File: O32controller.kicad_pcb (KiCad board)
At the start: 4 copper layers, 27 x 27 mm, 64 parts, among them J1 Conn_01x08_MountingPin, J2 BATT+, J3 BATT-, J4 Motor Connection, J5 Motor Connection, J6 Motor Connection, J7 BATT+, J8 BATT-, Q1 CSD88584Q5DCT, Q2 CSD88584Q5DCT, Q3 CSD88584Q5DCT, U1 AS5047D, U2 STSPIN32F0A

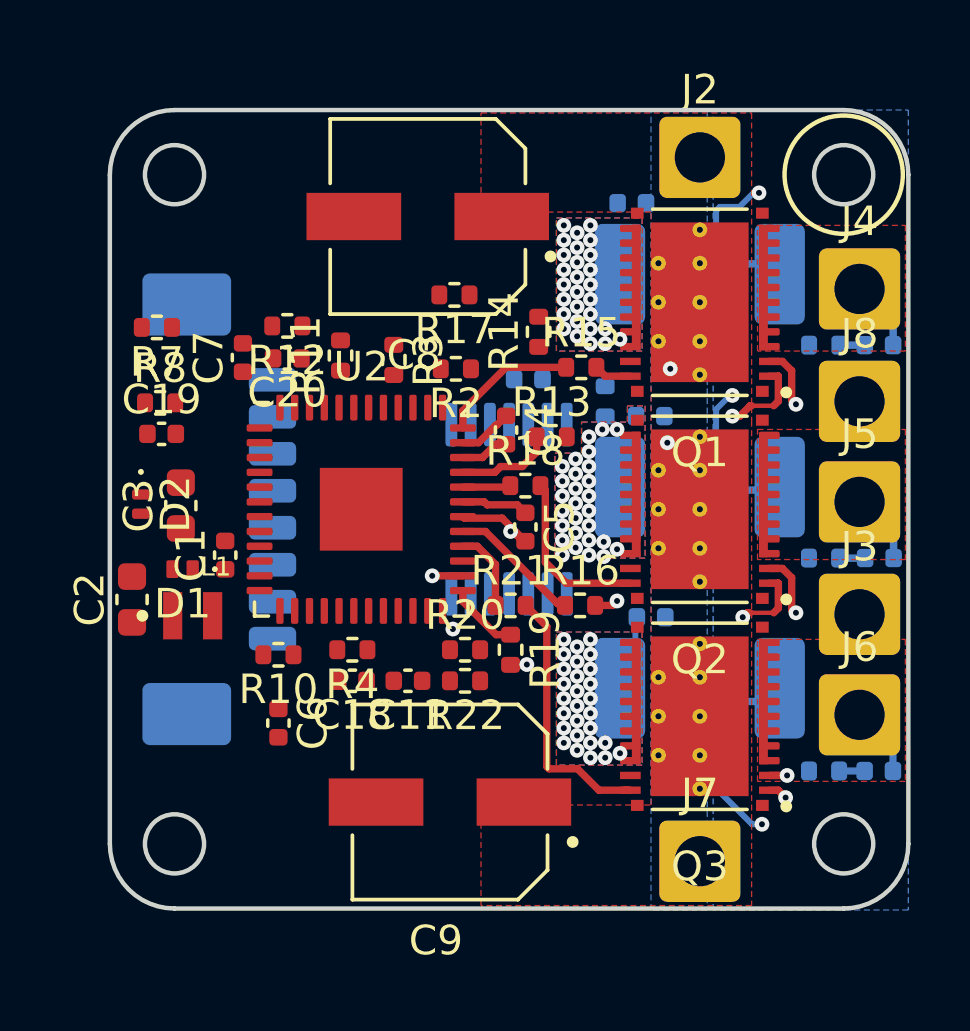
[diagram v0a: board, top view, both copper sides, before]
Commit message: fixed clearances
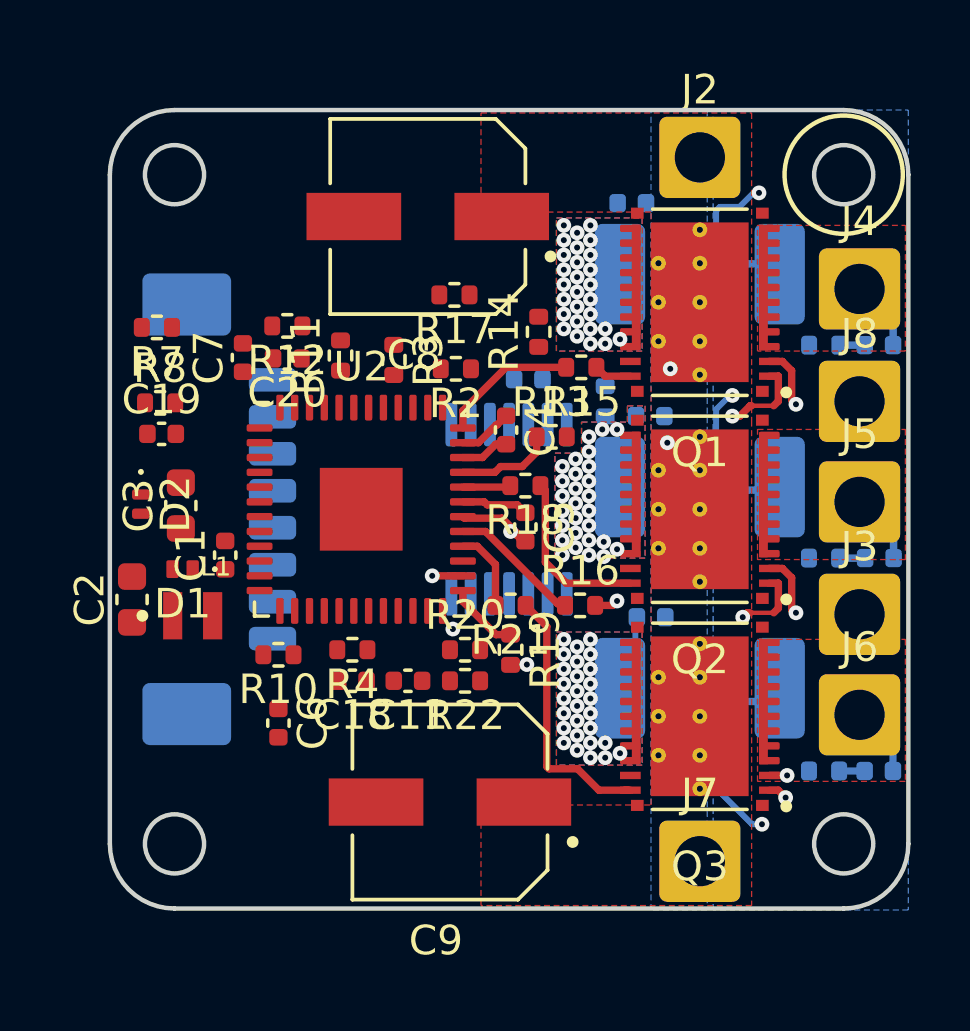
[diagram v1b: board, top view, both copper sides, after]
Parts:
- Q1, Q2, Q3: value CSD88584Q5DCT -> DMM0022A
- R1, R5, R9: value WFCP06124L000FE66 0.004R -> WSLF25122L000FEB 0.002R
- turned R15 to 180 degrees
- turned R18 to 180 degrees
- turned R21 to 180 degrees
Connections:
- R15 pad 1: /LSU -> /Motor phase U/GL_MOS
- R15 pad 2: /Motor phase U/GL_MOS -> /LSU
- R18 pad 1: /LSV -> /Motor phase V/GL_MOS
- R18 pad 2: /Motor phase V/GL_MOS -> /LSV
- R21 pad 1: /LSW -> /Motor phase W/GL_MOS
- R21 pad 2: /Motor phase W/GL_MOS -> /LSW
